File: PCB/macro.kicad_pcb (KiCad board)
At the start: 2 copper layers, 100 x 53 mm, 15 parts, among them SW1 SW_Push, SW2 SW_Push, SW3 SW_Push, SW5 SW_Push, SW8 SW_Push, SW9 SW_Push, U1 ESP32_DevKit_V1_DOIT, U3 COM-09032

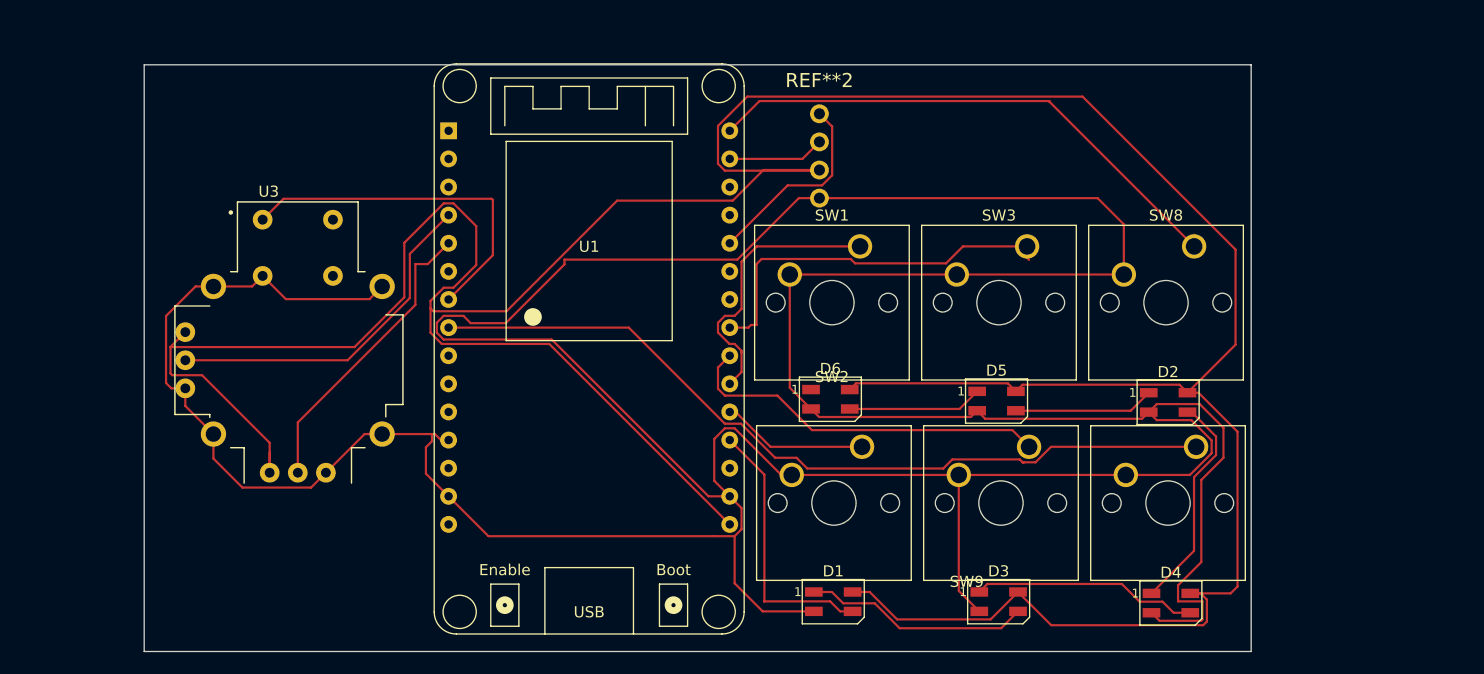
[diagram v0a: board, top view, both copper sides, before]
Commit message: Add files via upload
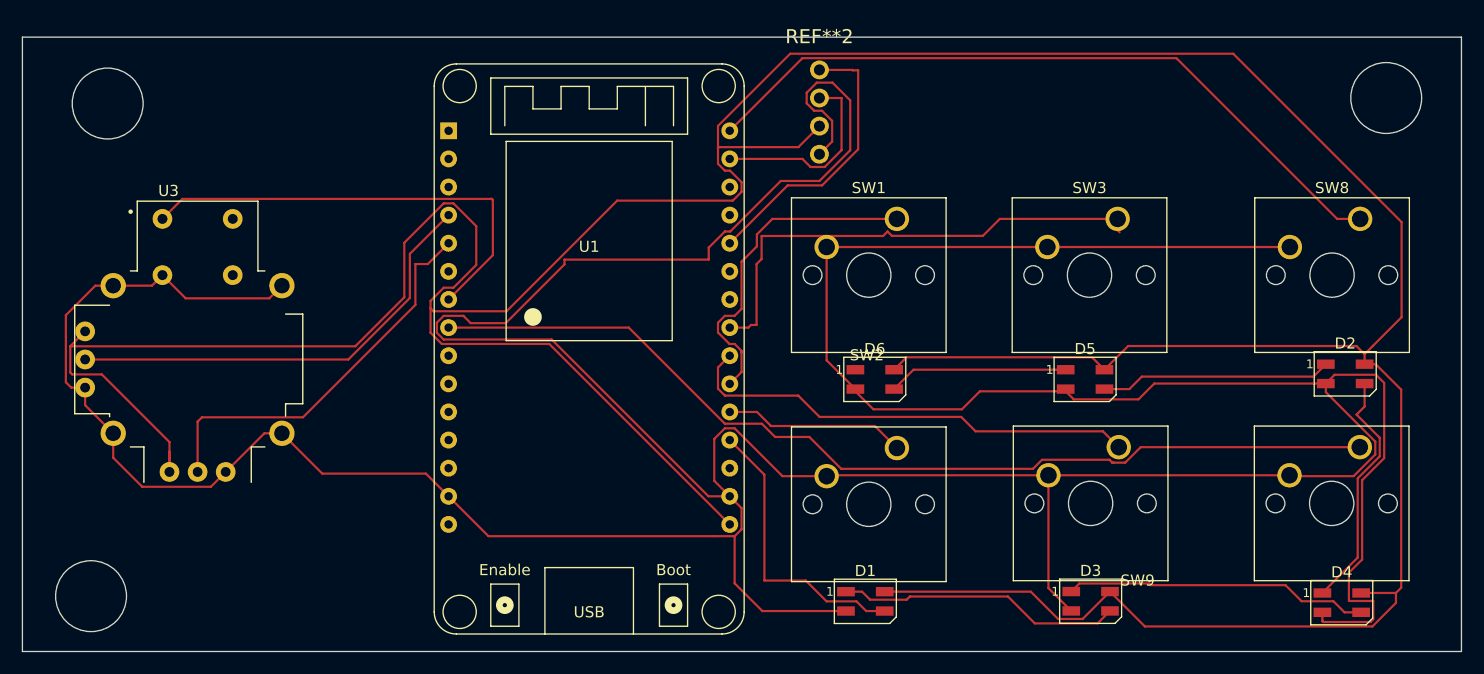
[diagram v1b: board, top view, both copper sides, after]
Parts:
- moved D2 16.2 mm to (226.0, 96.4)
- moved D4 15.4 mm to (225.7, 117.1)
- moved SW8 15.2 mm to (227.3, 82.4)
- moved SW9 14.8 mm to (227.3, 103.0)
- moved U3 9.05 mm to (122.3, 95.1)
- moved SW3 8.55 mm to (205.4, 82.4)
- moved D3 8.31 mm to (203.0, 117.0)
- moved D5 8.24 mm to (202.5, 96.9)
- moved SW5 8.10 mm to (205.5, 103.0)
- moved D6 4.39 mm to (183.5, 96.9)
- moved SW1 4.16 mm to (185.5, 82.4)
- moved REF**2 3.96 mm to (178.5, 69.0)
- moved SW2 3.15 mm to (185.5, 103.1)
- moved D1 2.90 mm to (182.6, 117.0)
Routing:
- net Net-(D1-VDD): track 320.1 -> 368.8 mm
- net GND: track 403.9 -> 442.8 mm
- net Net-(U1-IO23): track 49.6 -> 66.7 mm
- net Net-(U1-IO25): track 74.3 -> 89.1 mm
- net Net-(U1-IO5): track 34.3 -> 44.8 mm
- net Net-(U1-IO33): track 32.3 -> 41.4 mm
- net Net-(U1-IO35): track 27.0 -> 36.1 mm
- net Net-(U1-IO34): track 31.5 -> 40.6 mm
- net Net-(REF**2-SCL): track 8.74 -> 17.7 mm
- net Net-(D2-DOUT): track 12.7 -> 20.9 mm
- net Net-(U1-IO17): track 34.1 -> 42.2 mm
- net Net-(REF**2-SDA): track 17.8 -> 25.8 mm
- net Net-(D3-DOUT): track 20.4 -> 27.6 mm
- net Net-(D1-DOUT): track 20.4 -> 25.7 mm
- net Net-(U1-IO16): track 25.4 -> 30.4 mm
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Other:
- board size 100 x 53 mm -> 130 x 55.5 mm
